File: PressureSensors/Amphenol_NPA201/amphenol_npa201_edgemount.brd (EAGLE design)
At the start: 5 parts

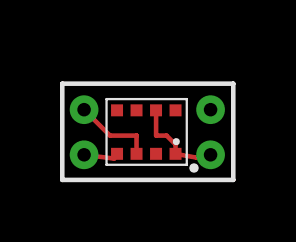
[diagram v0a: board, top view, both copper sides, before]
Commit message: overdue commit
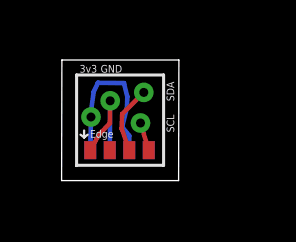
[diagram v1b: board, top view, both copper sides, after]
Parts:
- U$1: value AMPHENOL_NPA201 -> AMPHENOL_NPA201EDGEMOUNT; device Amphenol_NPA201:AMPHENOL_NPA201 -> Sombeck_lib:AMPHENOL_NPA201_EDGEMOUNT
- U$2, U$3, U$4, U$5: value WIREPAD_0,8/0,45 -> WIREPADWIREPAD_0,5/0,3; device wirepad_08-045:WIREPAD_0,8/0,45 -> Sombeck_lib:WIREPAD_0,5/0,3
- moved U$5 4.18 mm to (0.98, 2.12)
- moved U$4 3.36 mm to (1.62, 2.66)
- moved U$3 2.16 mm to (2.63, 1.92)
- moved U$2 2.07 mm to (2.74, 2.94), turned to 180 degrees
- moved U$1 1.60 mm to (1.93, 0.29), turned to 180 degrees
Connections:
- net +3V3: now also U$5.P$1; no longer U$4.P$1
- net GND: now also U$4.P$1; no longer U$5.P$1
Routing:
- net +3V3: track 0.00 -> 5.50 mm
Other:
- board outline added: 3.9 x 4 mm
- board text added: "3v3"
- board text added: "GND"
- board text added: "SCL"
- board text added: "SDA"
